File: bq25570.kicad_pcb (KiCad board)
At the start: 2 copper layers, 170.8 x 130.6 mm, 33 parts, among them J1 Conn_01x02_Male, J10 Conn_01x01_Male, J11 Conn_01x01_Male, J12 Conn_01x01_Male, J13 Conn_01x01_Male, J2 Conn_01x02_Male, J3 Conn_01x03_Male, J4 Conn_01x03_Male, J7 Conn_01x01_Male, J8 Conn_01x01_Male, J9 Conn_01x01_Male, U1 BQ25570

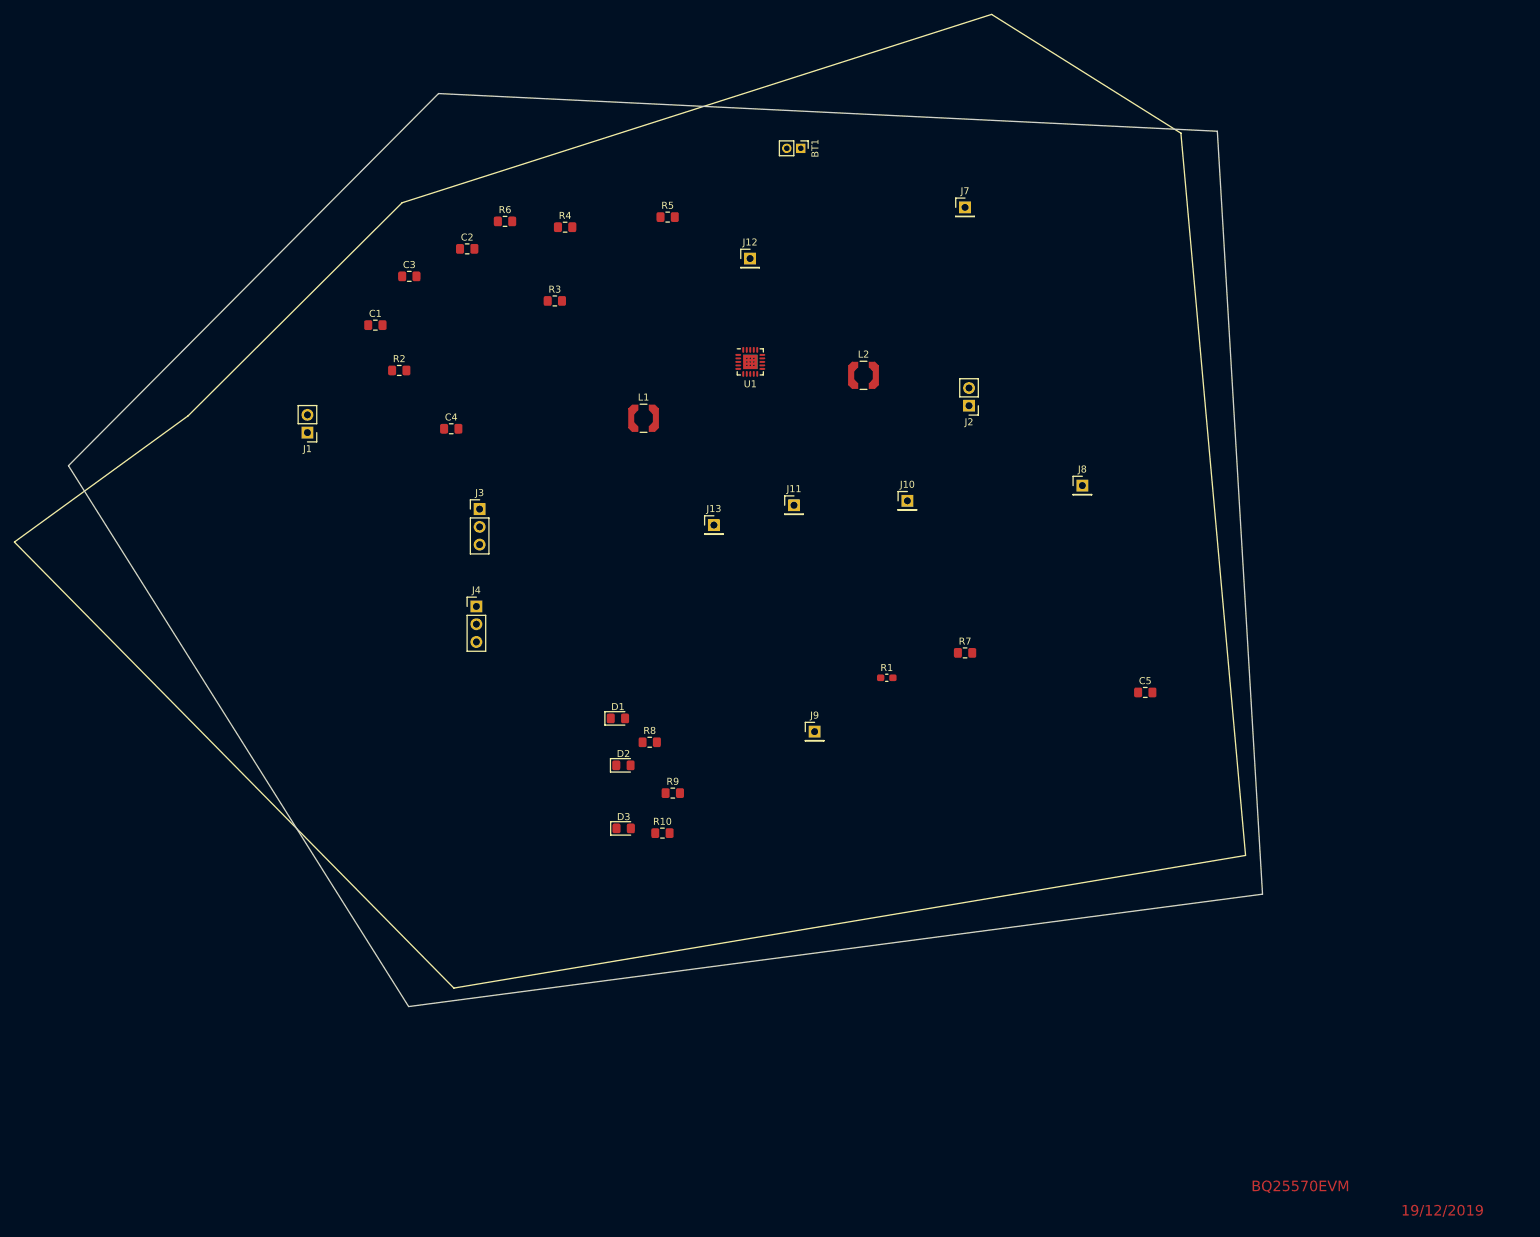
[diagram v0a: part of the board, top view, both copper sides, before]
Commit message: PCB started
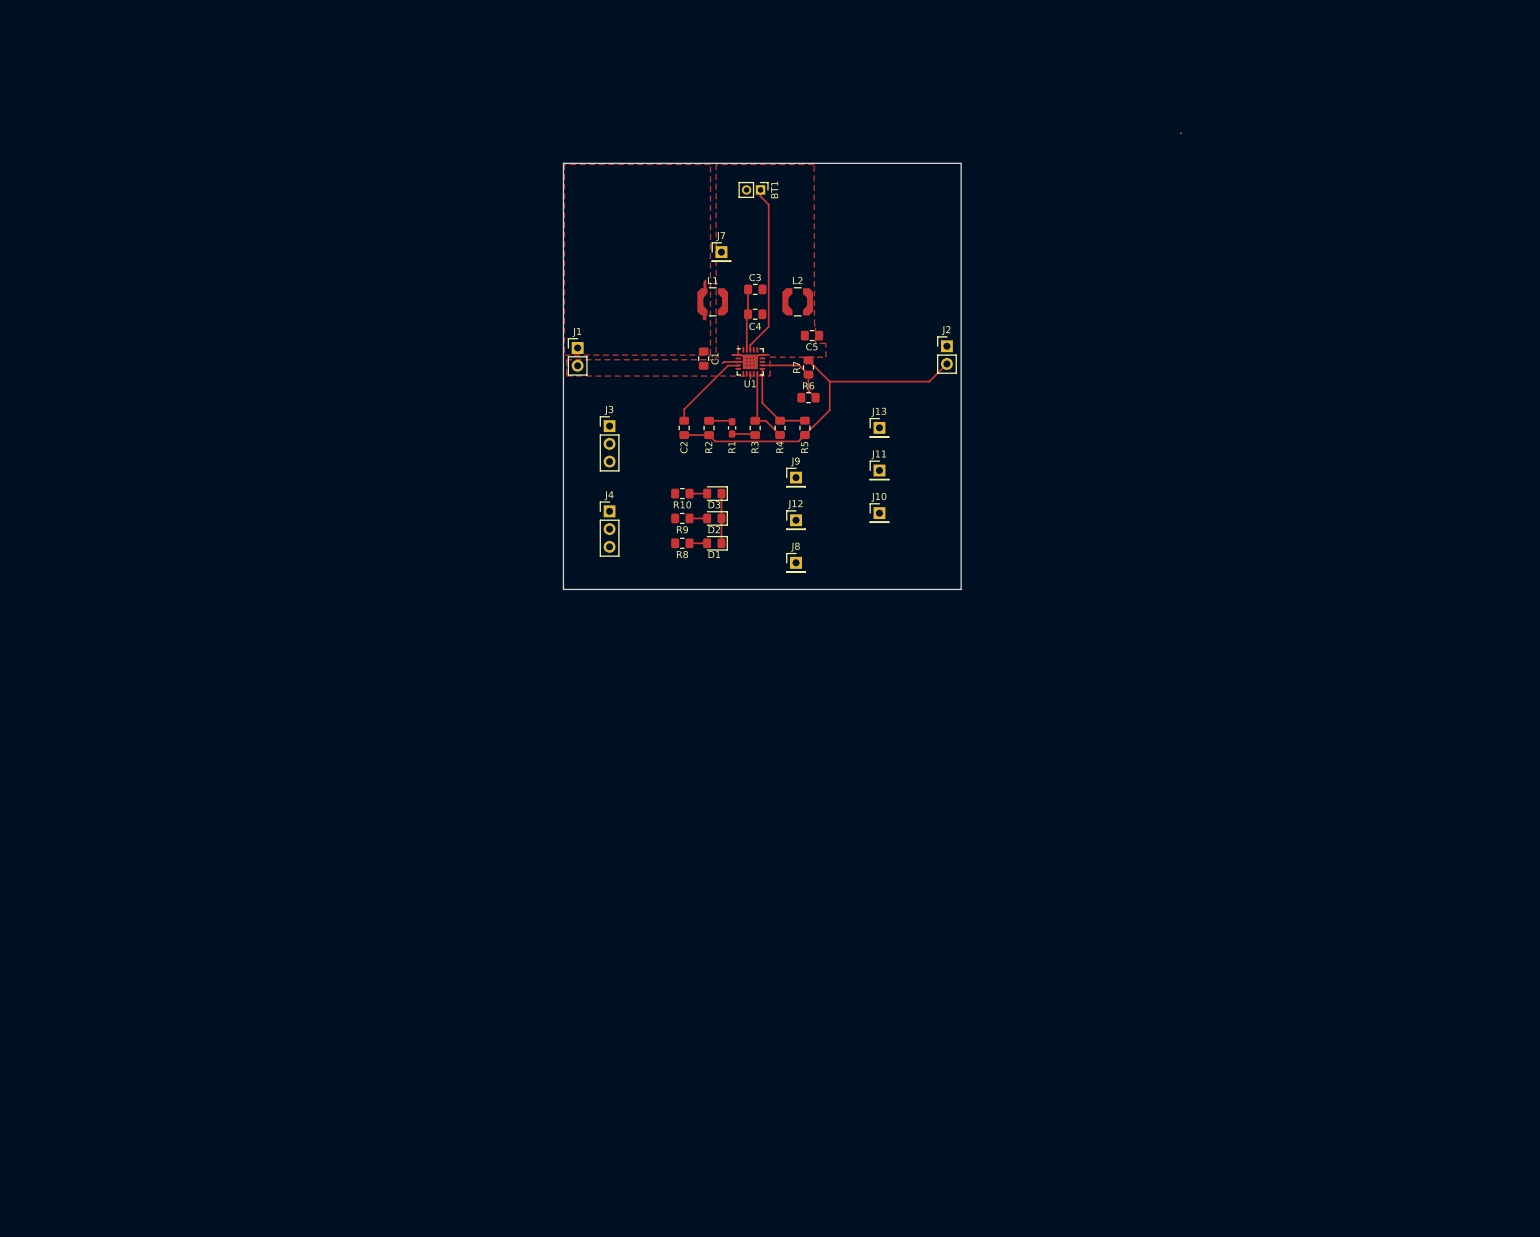
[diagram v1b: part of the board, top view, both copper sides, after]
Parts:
- moved C5 69.9 mm to (123.4, 67.8), turned to 180 degrees
- moved R6 50.2 mm to (122.9, 76.7)
- moved D3 49.6 mm to (109.5, 90.4), turned to 180 degrees
- moved C3 49.5 mm to (115.3, 61.2)
- moved R10 48.7 mm to (104.9, 90.4), turned to 180 degrees
- moved C1 47.2 mm to (108.0, 71.1), turned to 270 degrees
- moved R7 46.6 mm to (122.9, 72.4), turned to 90 degrees
- moved C4 46.5 mm to (115.3, 64.8)
- moved R2 45.1 mm to (108.7, 81.0), turned to 270 degrees
- moved J8 42.4 mm to (121.2, 100.3)
- moved R4 42.1 mm to (118.9, 81.0), turned to 90 degrees
- moved R1 42.0 mm to (112.0, 81.0), turned to 90 degrees
- moved J1 40.5 mm to (89.9, 69.6), turned to 0 degrees
- moved C2 40.2 mm to (105.2, 81.0), turned to 270 degrees
- moved R9 39.3 mm to (104.9, 94.0), turned to 180 degrees
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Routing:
- net /GND: track 0.00 -> 67.7 mm
- net /VBAT: track 0.00 -> 24.5 mm
- net /OK_PROG: track 0.00 -> 12.0 mm
- net /VREF_SAMP: track 0.00 -> 12.0 mm
- net /OK_HYST: track 0.00 -> 11.2 mm
- net /VOUT_SET: track 0.00 -> 10.9 mm
- net /VSTOR: track 0.00 -> 8.73 mm
- net /VIN_DC: track 0.00 -> 5.33 mm
- net /VRDIV: track 0.00 -> 4.04 mm
- net /VBAT_OV: track 0.00 -> 3.36 mm
- net Net-(D3-Pad2): track 0.00 -> 2.52 mm
- net Net-(D2-Pad2): track 0.00 -> 2.52 mm
- net Net-(D1-Pad2): track 0.00 -> 2.52 mm
- net /LBUCK: track 0.00 -> 1.65 mm
- added copper zone on F.Cu, net /GND
- added copper zone on F.Cu, net /VIN_DC
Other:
- board size 170.8 x 130.6 mm -> 56.9 x 61 mm
- board text removed: "19/12/2019"
- board text removed: "BQ25570EVM"
